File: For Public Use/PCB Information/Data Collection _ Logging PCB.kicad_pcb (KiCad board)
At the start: 2 copper layers, 35.6 x 53.3 mm, 8 parts, among them U1 TC2014-3.3VxCTTR

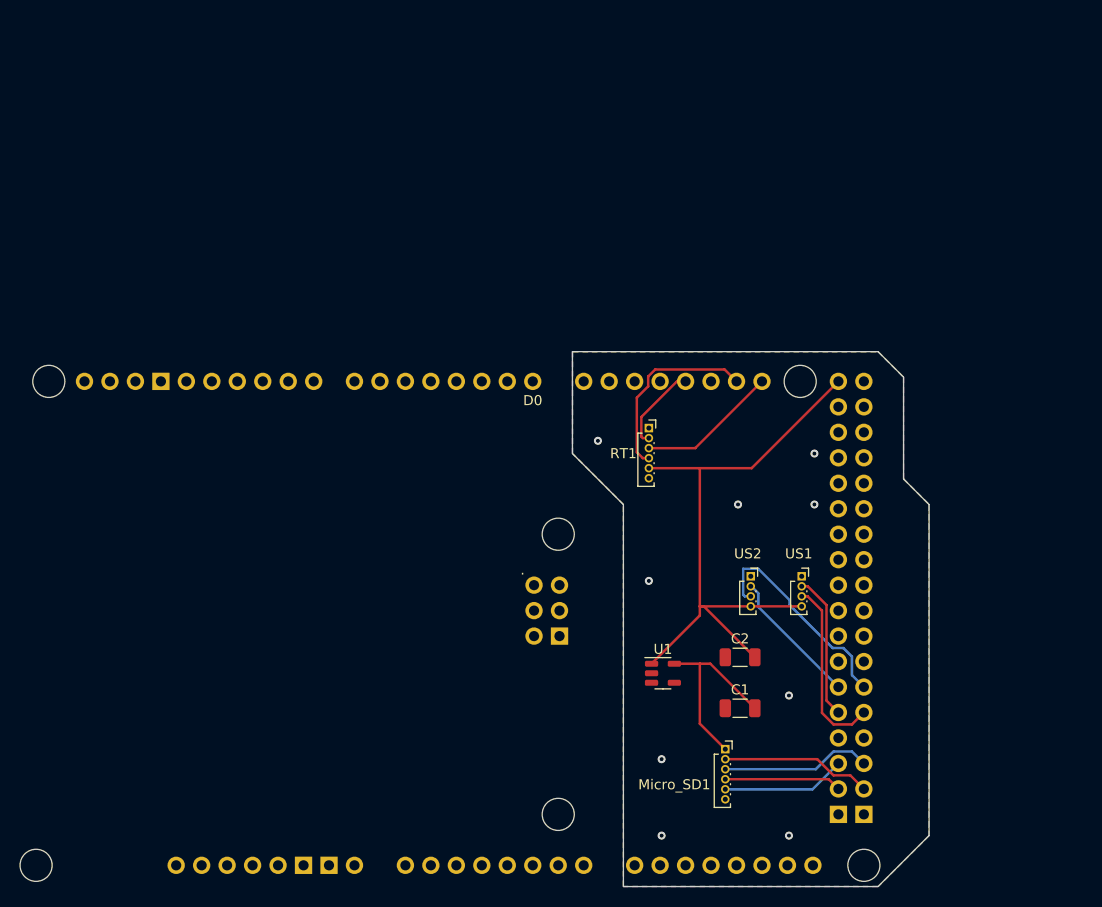
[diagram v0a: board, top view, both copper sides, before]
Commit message: Redid the current PCB Information
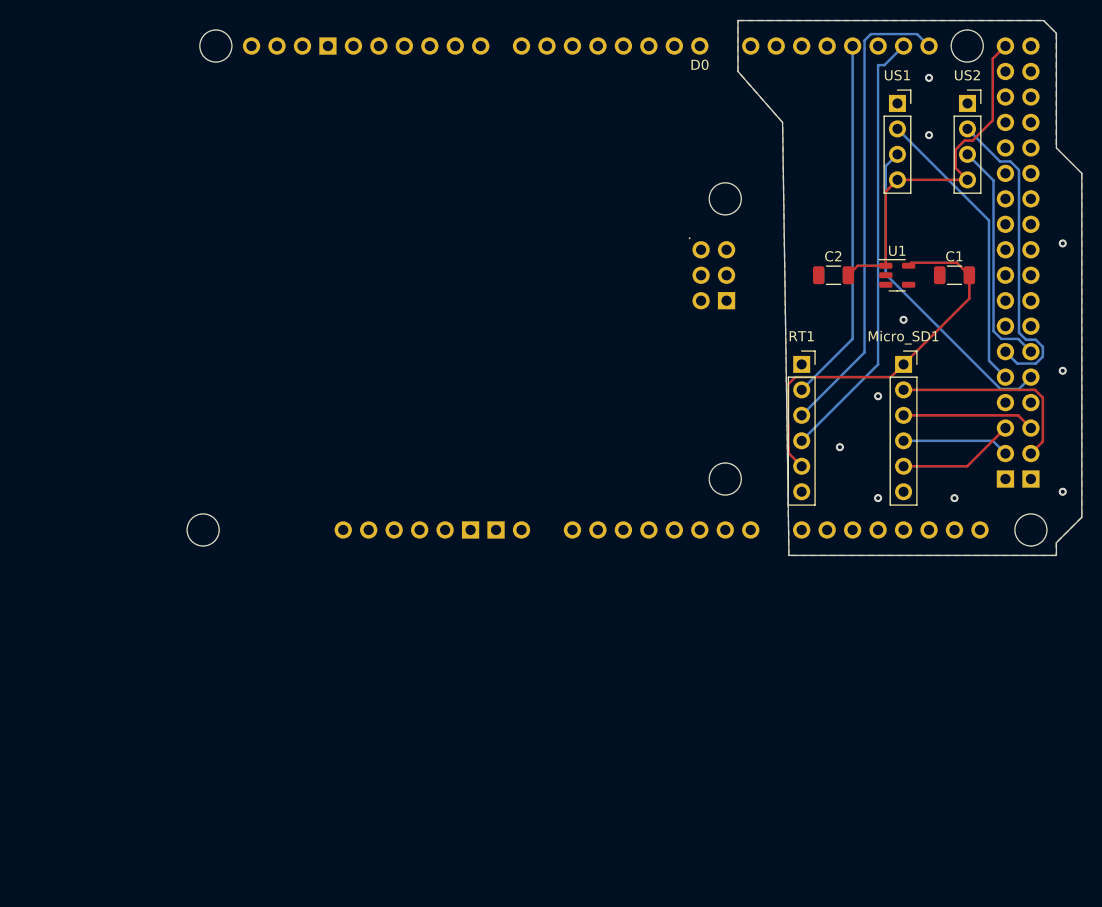
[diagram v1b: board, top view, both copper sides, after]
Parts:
- Micro_SD1, RT1: footprint Connector_PinSocket_1.00mm:PinSocket_1x06_P1.00mm_Vertical -> Connector_PinSocket_2.54mm:PinSocket_1x06_P2.54mm_Vertical
- US1, US2: footprint Connector_PinSocket_1.00mm:PinSocket_1x04_P1.00mm_Vertical -> Connector_PinSocket_2.54mm:PinSocket_1x04_P2.54mm_Vertical
- moved US2 51.9 mm to (194.3, 81.9)
- moved C1 48.2 mm to (193.0, 99.1)
- moved US1 48.1 mm to (187.3, 81.9)
- moved U1 46.1 mm to (187.3, 99.1)
- moved Micro_SD1 42.3 mm to (188.0, 108.0)
- moved C2 39.2 mm to (181.0, 99.1)
- moved XA1 37.4 mm to (104.1, 127.0)
- moved RT1 16.5 mm to (177.8, 108.0)
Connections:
- C2 pad 2: Net-(RT1-VCC) -> Net-(U1-VIN)
- RT1 pad 5: Net-(RT1-VCC) -> Net-(Micro_SD1-3.3V)
- U1 pad 1: Net-(RT1-VCC) -> Net-(U1-VIN)
- US1 pad 4: Net-(RT1-VCC) -> Net-(U1-VIN)
- US2 pad 4: Net-(RT1-VCC) -> Net-(U1-VIN)
- XA1 pad 5V3: Net-(RT1-VCC) -> Net-(U1-VIN)
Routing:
- net Net-(RT1-VCC): track 61.7 -> 0.00 mm
- net Net-(U1-VIN): track 0.00 -> 36.5 mm
- net Net-(RT1-SCL): track 14.0 -> 47.2 mm
- net Net-(RT1-~{INT}/SQW): track 8.65 -> 36.4 mm
- net Net-(RT1-SDA): track 19.1 -> 44.0 mm
- net Net-(Micro_SD1-3.3V): track 19.4 -> 39.3 mm
- net Net-(US2-ECHO): track 13.7 -> 31.5 mm
- net Net-(US1-ECHO): track 14.5 -> 29.2 mm
- net Net-(US1-TRIG): track 18.0 -> 32.2 mm
- net Net-(Micro_SD1-CS): track 15.0 -> 20.3 mm
- net Net-(Micro_SD1-MOSI): track 15.0 -> 13.2 mm
- net Net-(US2-TRIG): track 21.7 -> 23.3 mm
- net Net-(Micro_SD1-CLK): track 11.7 -> 10.7 mm
- net Net-(Micro_SD1-MISO): track 12.3 -> 11.7 mm
- net GND: vias 9 -> 10
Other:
- board size 35.6 x 53.3 mm -> 34.3 x 53.3 mm
- board text added: "Datalogging v0.2 5/16/2024 Nicholas Liger ARTS Lab - USC"
- board text removed: "Datalogging Board v1.0 5/10/2024 Nicholas Liger ARTS Lab - USC"
